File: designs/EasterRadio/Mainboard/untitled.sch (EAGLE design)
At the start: 67 parts, among them IC1 74HC595D, IC2 74HC595D, IC3 74HC595D, IC4 Analog Digital

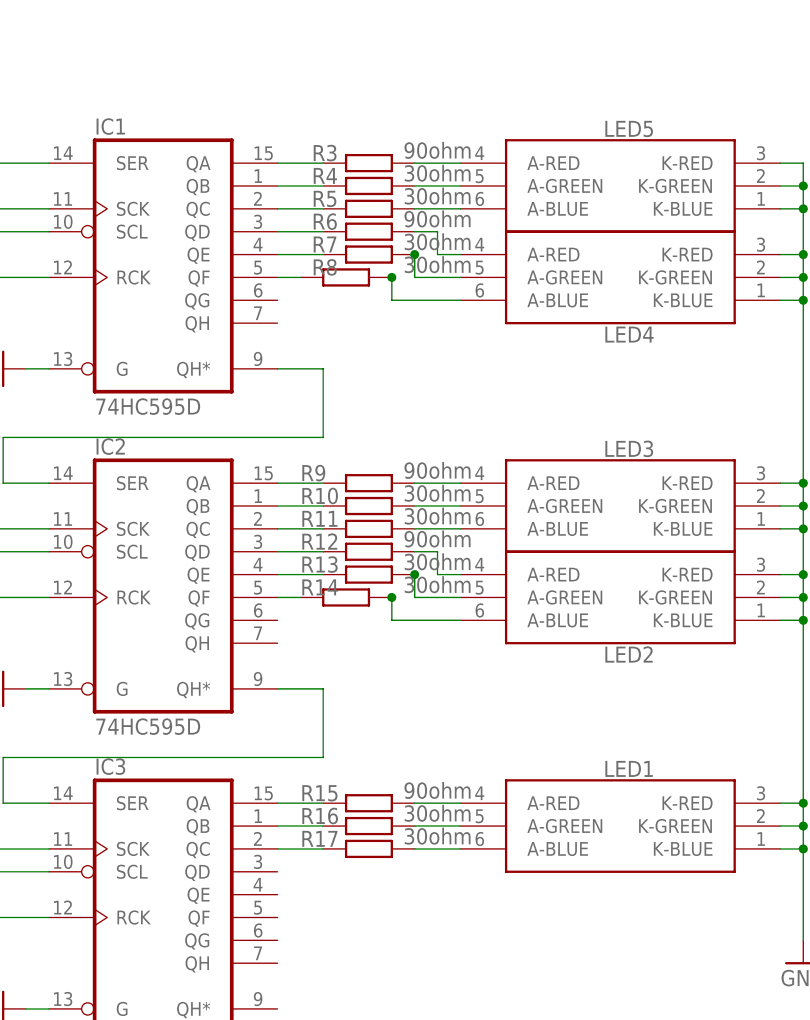
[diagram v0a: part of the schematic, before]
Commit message: added new mainboard design
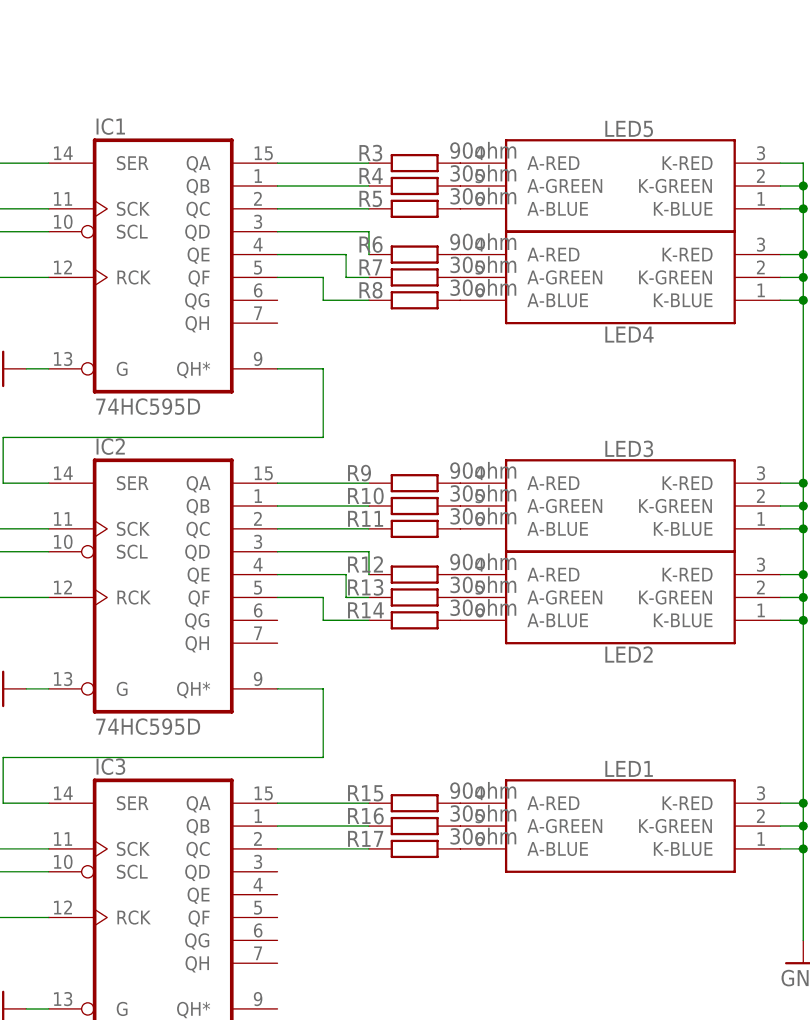
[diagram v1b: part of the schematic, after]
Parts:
- R1, R2: device rcl:R-EU_R0805 -> rcl:R-EU_R0603
- R10, R11, R12, R13, R14, R15, R16, R17, R3, R4, R5, R6, R7, R8, R9: device rcl:R-EU_R0805 -> rcl:R-EU_R0402
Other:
- moved on the sheet: R10, R11, R12, R13, R14, R15, R16, R17, R3, R4, R5, R6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
